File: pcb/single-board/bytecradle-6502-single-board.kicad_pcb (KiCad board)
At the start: 2 copper layers, 55 parts, among them J2 USB_B, J3 Serial, SW1 SW_DIP_x04, SW2 RESET, SW3 NMI, U1 W65C02SxP, U10 74HC688, U11 74HC32, U12 74HC688, U13 W65C22NxP, U14 74HC193, U15 74HC193, U16 74HC14, U17 74HC688, U18 74HC00, U2 SST39SF040, U3 74HC273, U4 74HC688, U5 W65C51NxP, U6 74HC00, U7 CY62256-70PC, U8 CY62256-70PC, U9 74HC245, X1 32MHz, Y1 Crystal

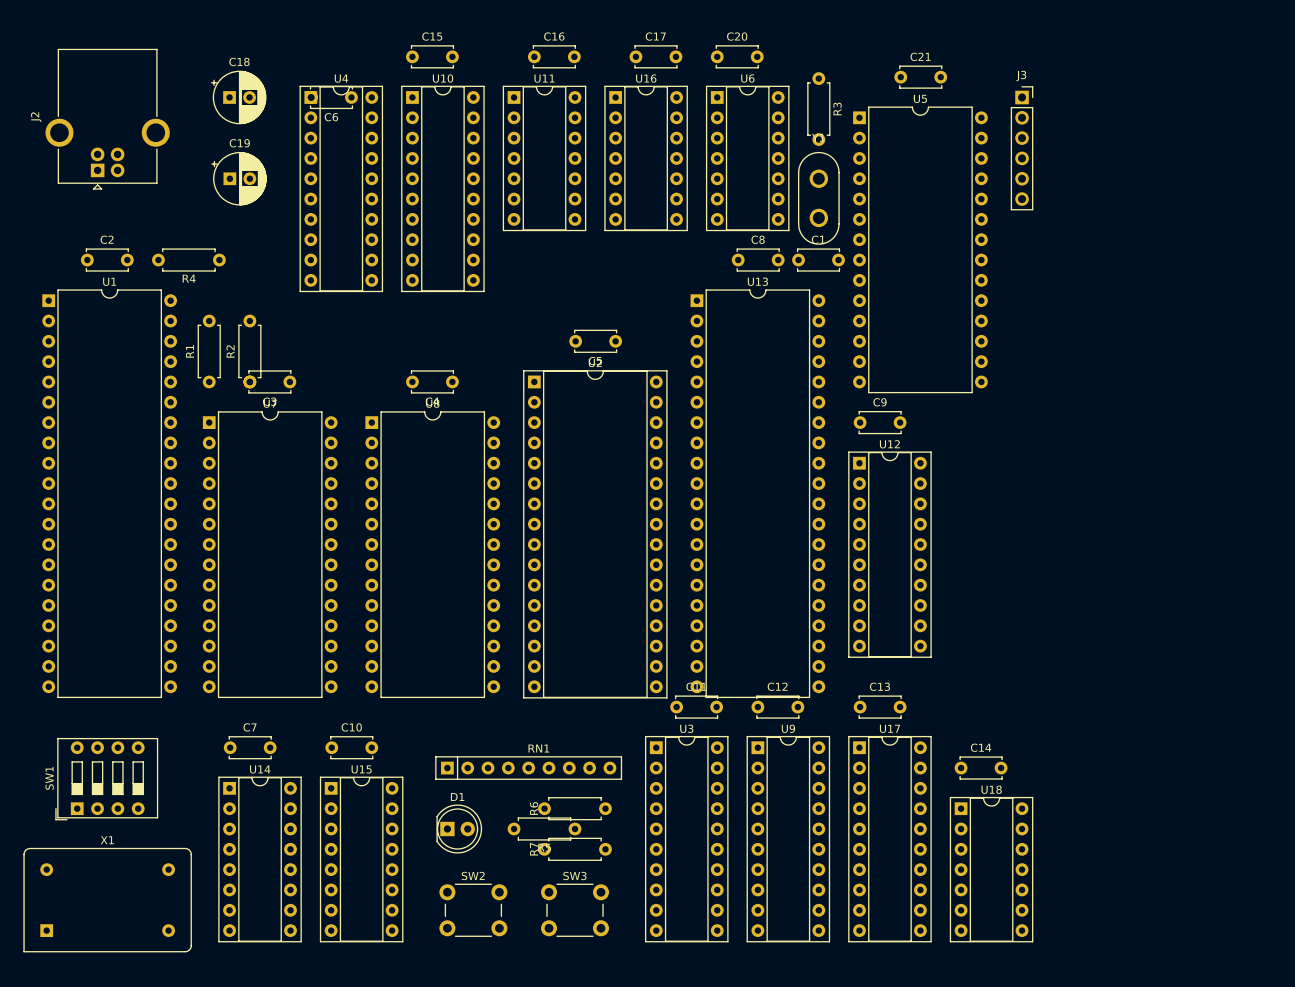
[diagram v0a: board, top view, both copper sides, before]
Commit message: Tuning design
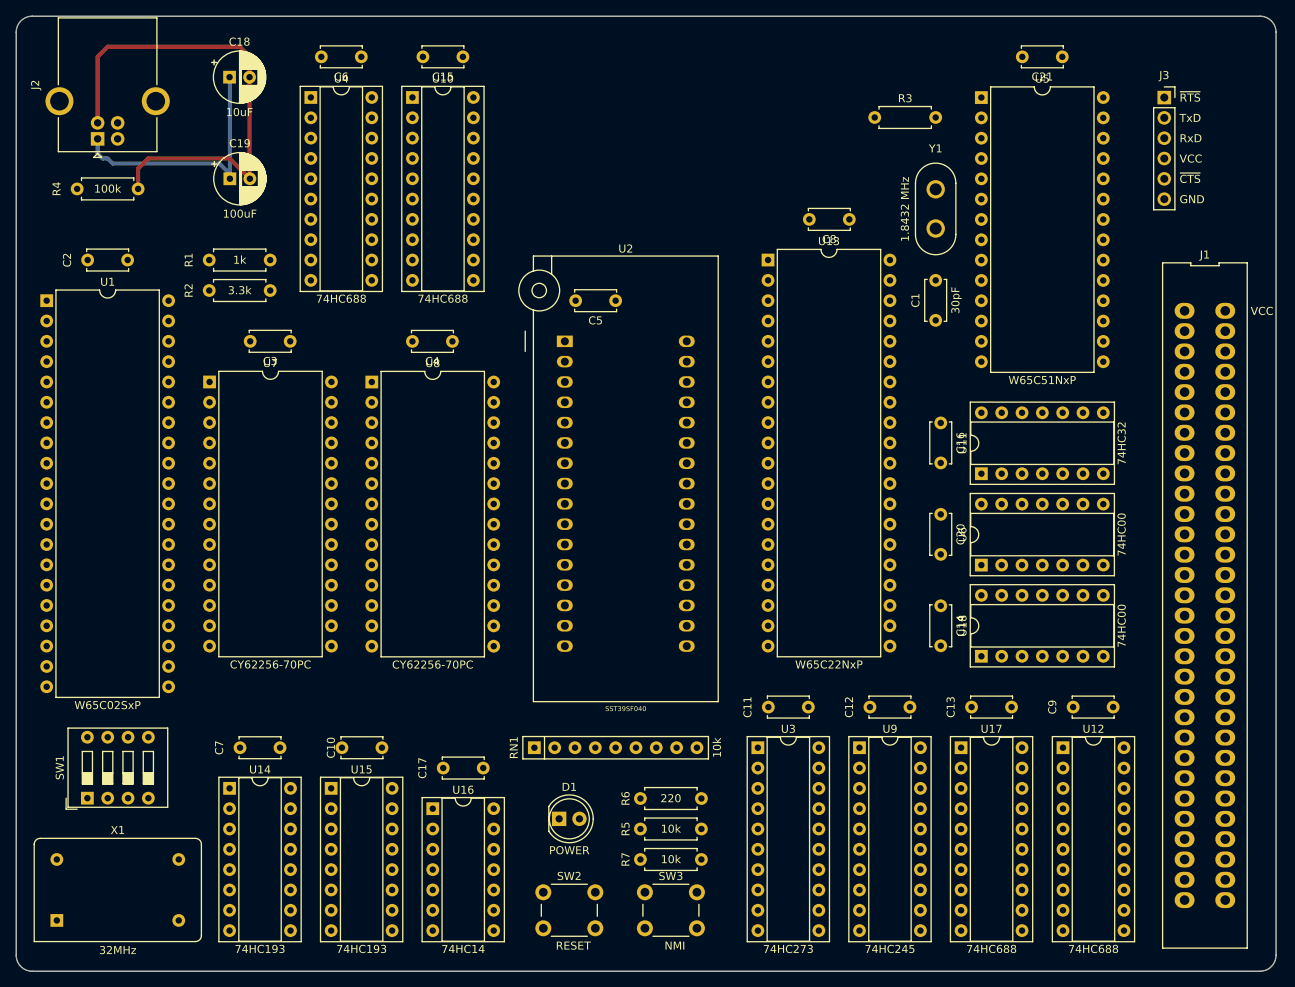
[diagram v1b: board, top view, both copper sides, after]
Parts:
- added J1: BUS, edgeconn:DIP-60_200_ELL, F.Cu at (170.2, 114.3)
- RN1: value R_Network08 -> 10k
- U2: footprint Package_DIP:DIP-32_W15.24mm_Socket -> Socket:DIP_Socket-32_W11.9_W12.7_W15.24_W17.78_W18.5_3M_232-1285-00-0602J
- Y1: value Crystal -> 1.8432 MHz
- moved U16 91.8 mm to (73.7, 139.7)
- moved C17 90.9 mm to (80.0, 134.6), turned to 180 degrees
- moved U11 75.0 mm to (142.2, 97.8), turned to 90 degrees
- moved C16 68.4 mm to (137.2, 91.5), turned to -90 degrees
- moved U6 67.1 mm to (142.2, 109.2), turned to 90 degrees
- moved C20 63.7 mm to (137.2, 102.9), turned to -90 degrees
- moved C9 47.6 mm to (158.7, 127.0), turned to 180 degrees
- moved U12 43.7 mm to (152.4, 132.1)
- moved C14 20.4 mm to (137.2, 114.3), turned to -90 degrees
- moved C21 20.4 mm to (152.4, 45.7), turned to 180 degrees
- moved U18 19.2 mm to (142.2, 120.7), turned to 90 degrees
- moved C12 19.0 mm to (133.3, 127.0), turned to 180 degrees
- moved C13 18.9 mm to (146.0, 127.0), turned to 180 degrees
- moved C1 18.7 mm to (136.5, 78.7), turned to 90 degrees
- moved J3 17.8 mm to (165.1, 50.8)
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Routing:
- net GND: track 0.00 -> 61.7 mm
- net VCC: track 0.00 -> 32.7 mm
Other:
- board outline added: 157.5 x 119.4 mm
- board text added: "GND"
- board text added: "RxD"
- board text added: "TxD"
- board text added: "VCC"
- board text added: "~{CTS}"
- board text added: "~{RTS}"

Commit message: Adding details
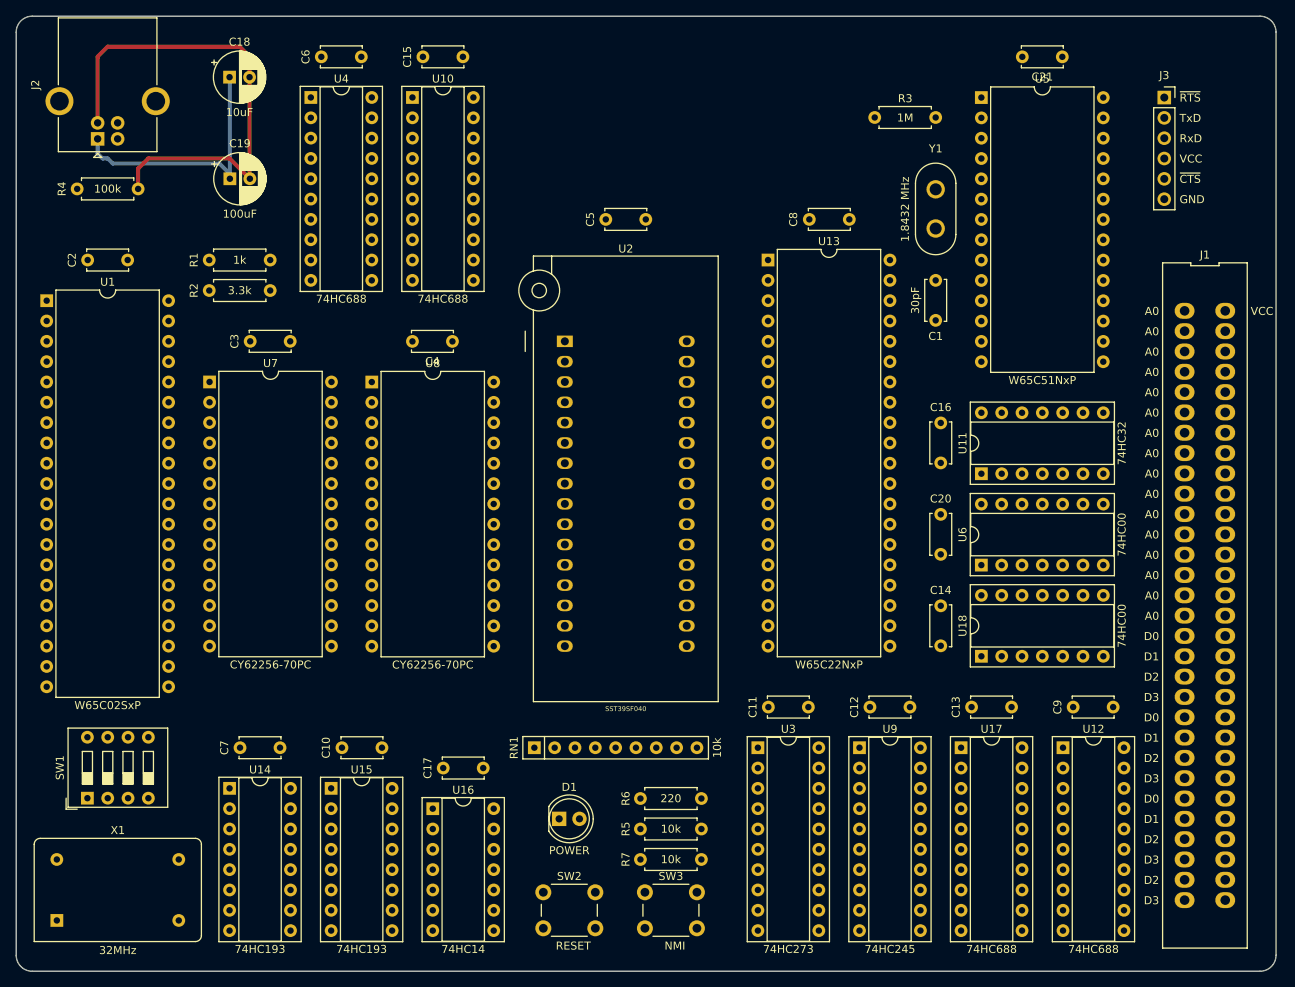
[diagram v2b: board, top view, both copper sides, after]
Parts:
- moved C5 10.8 mm to (100.3, 66.0)
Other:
- board text added: "A0"
- board text added: "D0"
- board text added: "D1"
- board text added: "D2"
- board text added: "D3"

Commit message: Pre-routing commit
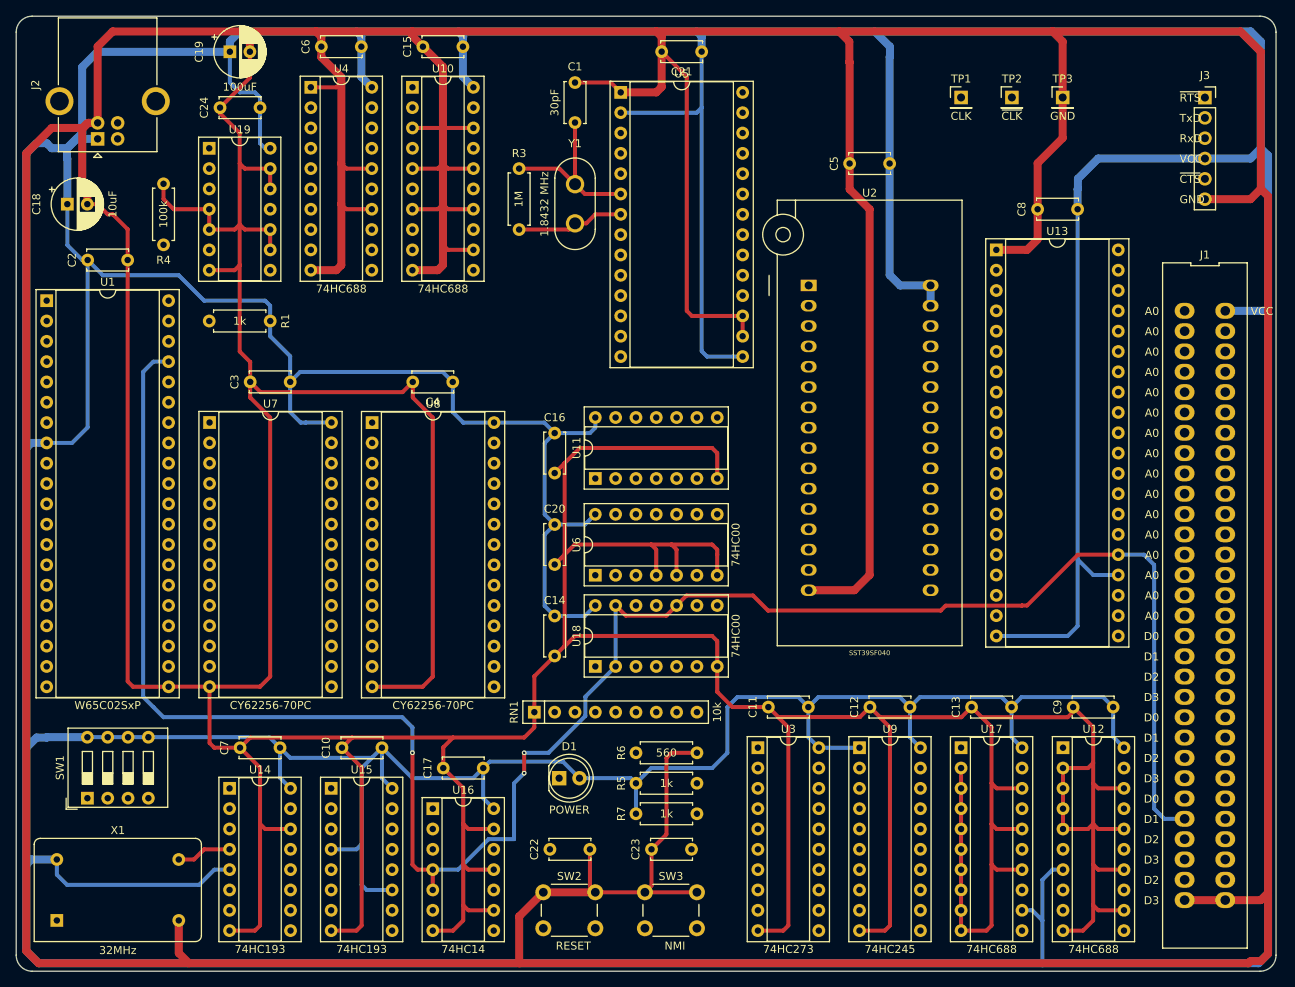
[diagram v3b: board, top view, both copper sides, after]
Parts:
- removed R2: 3.3k, Resistor_THT:R_Axial_DIN0207_L6.3mm_D2.5mm_P7.62mm_Horizontal
- added C22: 100nF, Capacitor_THT:C_Disc_D5.0mm_W2.5mm_P5.00mm, F.Cu at (88.3, 144.8)
- added C23: 100nF, Capacitor_THT:C_Disc_D5.0mm_W2.5mm_P5.00mm, F.Cu at (106.0, 144.8)
- added C24: 100nF, Capacitor_THT:C_Disc_D5.0mm_W2.5mm_P5.00mm, F.Cu at (52.1, 52.1)
- added TP1: CLK, Connector_PinHeader_2.54mm:PinHeader_1x01_P2.54mm_Vertical, F.Cu at (139.7, 50.8)
- added TP2: ~{CLK}, Connector_PinHeader_2.54mm:PinHeader_1x01_P2.54mm_Vertical, F.Cu at (146.1, 50.8)
- added TP3: GND, Connector_PinHeader_2.54mm:PinHeader_1x01_P2.54mm_Vertical, F.Cu at (152.4, 50.8)
- added U19: 74HC08, Package_DIP:DIP-14_W7.62mm_Socket, F.Cu at (45.7, 57.1)
- R5, R7: value 10k -> 1k
- R6: value 220 -> 560
- U1, U13: footprint Package_DIP:DIP-40_W15.24mm -> Package_DIP:DIP-40_W15.24mm_Socket
- U11: value 74HC32 -> 74HC02
- U5, U7, U8: footprint Package_DIP:DIP-28_W15.24mm -> Package_DIP:DIP-28_W15.24mm_Socket
- moved C1 54.0 mm to (91.4, 48.9), turned to -90 degrees
- moved U6 48.3 mm to (94.0, 110.5)
- moved U18 48.3 mm to (94.0, 121.9)
- moved C14 48.3 mm to (88.9, 115.6)
- moved C16 48.3 mm to (88.9, 92.8)
- moved C20 48.3 mm to (88.9, 104.2)
- moved U11 48.3 mm to (94.0, 98.4)
- moved U5 45.1 mm to (97.2, 50.2)
- moved Y1 45.1 mm to (91.4, 66.5)
- moved C21 45.1 mm to (107.3, 45.1)
- moved R3 44.9 mm to (84.5, 59.7), turned to -90 degrees
- moved C5 31.3 mm to (130.8, 59.1)
- moved U2 31.3 mm to (120.7, 74.3)
- moved U13 28.6 mm to (144.1, 69.8)
- moved C8 28.6 mm to (154.3, 64.8)
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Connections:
- U11 pad 1: ~{R}/W -> Net-(U8-~{OE})
- U11 pad 11: unconnected-(U11-Pad11) -> Net-(U10-P=R)
- U11 pad 12: GND -> Net-(U10-P=R)
- U11 pad 13: GND -> Net-(U11-Pad13)
- U11 pad 2: Net-(U10-P=R) -> Net-(U11-Pad2)
- U11 pad 3: Net-(U9-CE) -> Net-(U11-Pad2)
- U11 pad 4: R/~{W} -> Net-(U11-Pad2)
- U11 pad 5: Net-(U10-P=R) -> Net-(U11-Pad5)
- U11 pad 6: Net-(U11-Pad6) -> A14
- U11 pad 8: Net-(U8-~{CS}) -> R/~{W}
- U11 pad 9: A14 -> Net-(U10-P=R)
- U13 pad 21: ~{IRQ} -> ~{IRQC22}
- U16 pad 5: GND -> CLK
- U16 pad 6: unconnected-(U16-Pad6) -> ~{CLK}
- U18 pad 1: Net-(U18-Pad1) -> Net-(U11-Pad10)
- U18 pad 10: GND -> CLK
- U18 pad 11: unconnected-(U18-Pad11) -> Net-(U7-~{CS})
- U18 pad 12: GND -> Net-(U18-Pad12)
- U18 pad 13: GND -> CLK
- U18 pad 4: Net-(U11-Pad6) -> Net-(U11-Pad13)
- U18 pad 5: Net-(U11-Pad6) -> R/~{W}
- U18 pad 6: Net-(U18-Pad1) -> Net-(U9-CE)
- U18 pad 8: unconnected-(U18-Pad8) -> Net-(U8-~{CS})
- U18 pad 9: GND -> Net-(U11-Pad2)
- U2 pad 24: ~{R}/W -> Net-(U2-CE)
- U5 pad 26: ~{IRQ} -> ~{IRQC51}
- U6 pad 11: Net-(U7-~{WE}) -> Net-(U18-Pad12)
- U6 pad 12: ~{R}/W -> A15
- U6 pad 13: CLK -> A15
- U6 pad 4: R/~{W} -> GND
- U6 pad 5: R/~{W} -> GND
- U6 pad 6: ~{R}/W -> unconnected-(U6-Pad6)
- U6 pad 8: Net-(U11-Pad10) -> Net-(U11-Pad5)
- U7 pad 20: A15 -> Net-(U7-~{CS})
- U7 pad 22: ~{R}/W -> A15
- U7 pad 27: Net-(U7-~{WE}) -> R/~{W}
- U8 pad 22: ~{R}/W -> Net-(U8-~{OE})
- U8 pad 27: Net-(U7-~{WE}) -> R/~{W}
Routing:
- net GND: track 61.7 -> 1684.4 mm
- net VCC: track 32.7 -> 1214.4 mm
- net CLK: track 0.00 -> 257.9 mm, vias 0 -> 3
- net Net-(U5-XTAL1): track 0.00 -> 21.7 mm
- net Net-(U5-XTAL2): track 0.00 -> 13.5 mm
- net Net-(U14-DOWN): track 0.00 -> 6.88 mm
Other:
- copper layers 2 -> 4
